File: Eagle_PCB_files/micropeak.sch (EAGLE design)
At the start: 10 parts, among them U1 ATTINY85-20MUR, U2 MS5611-01BA03

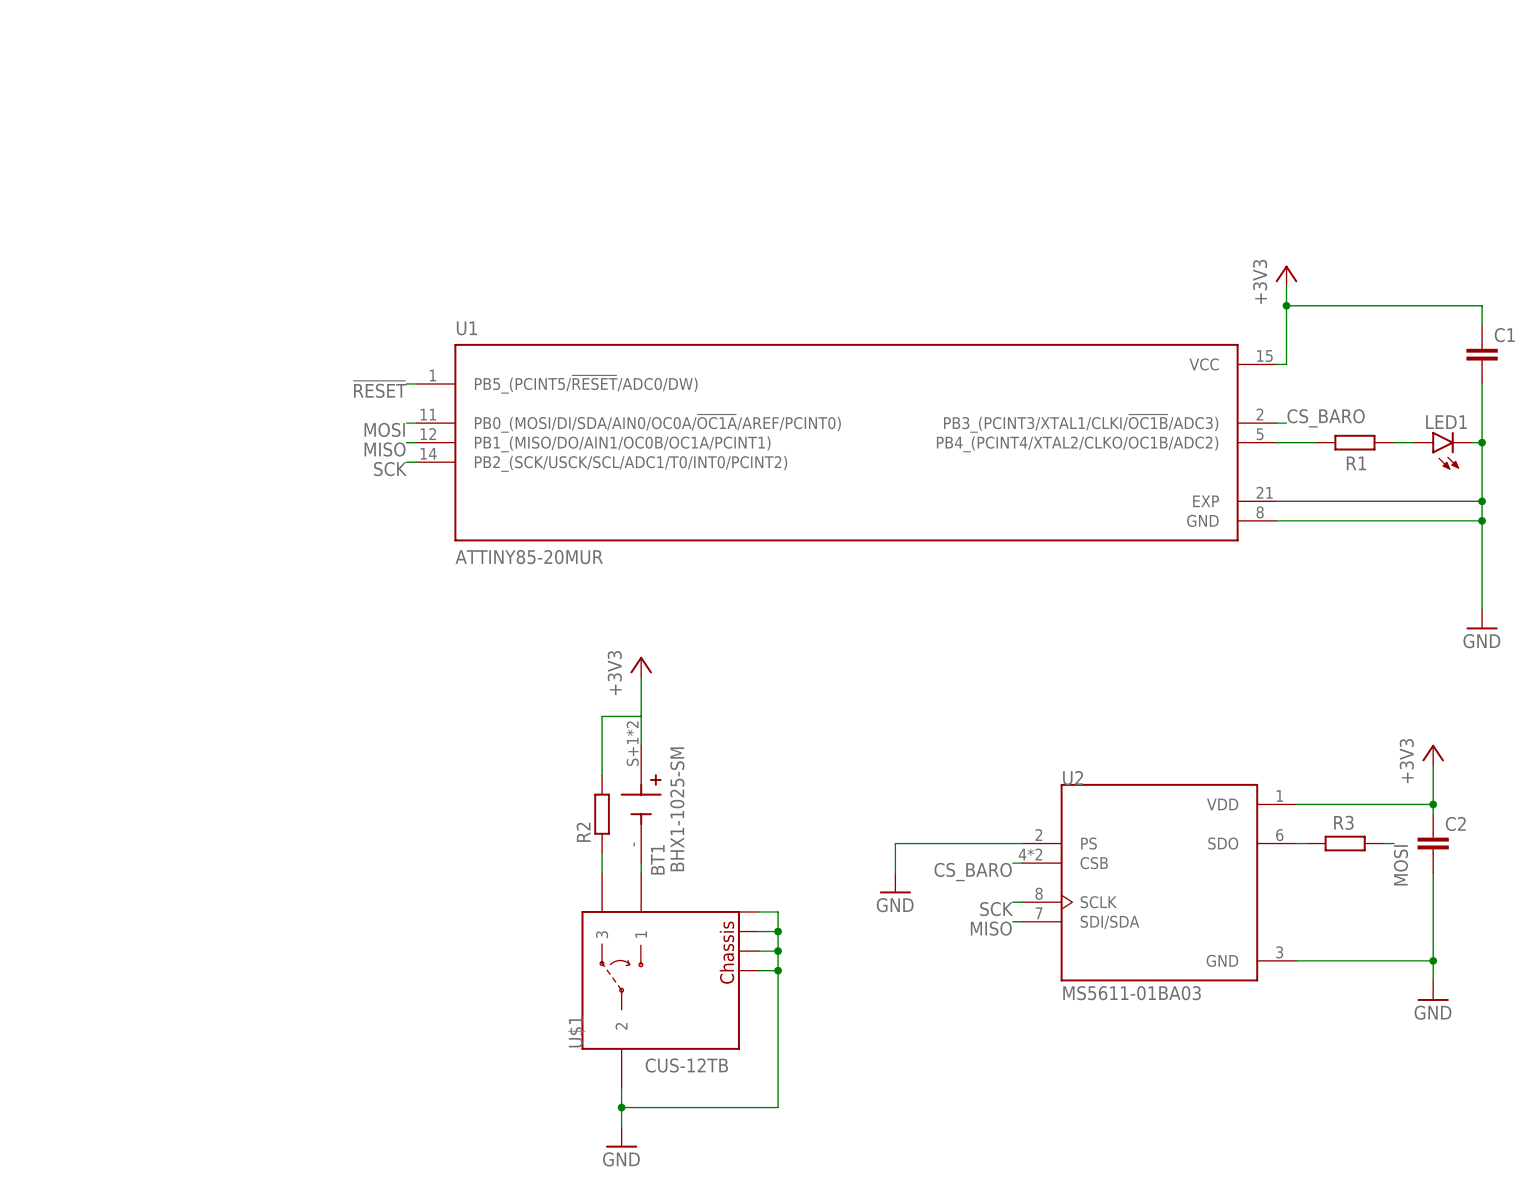
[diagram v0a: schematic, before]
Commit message: schematic done
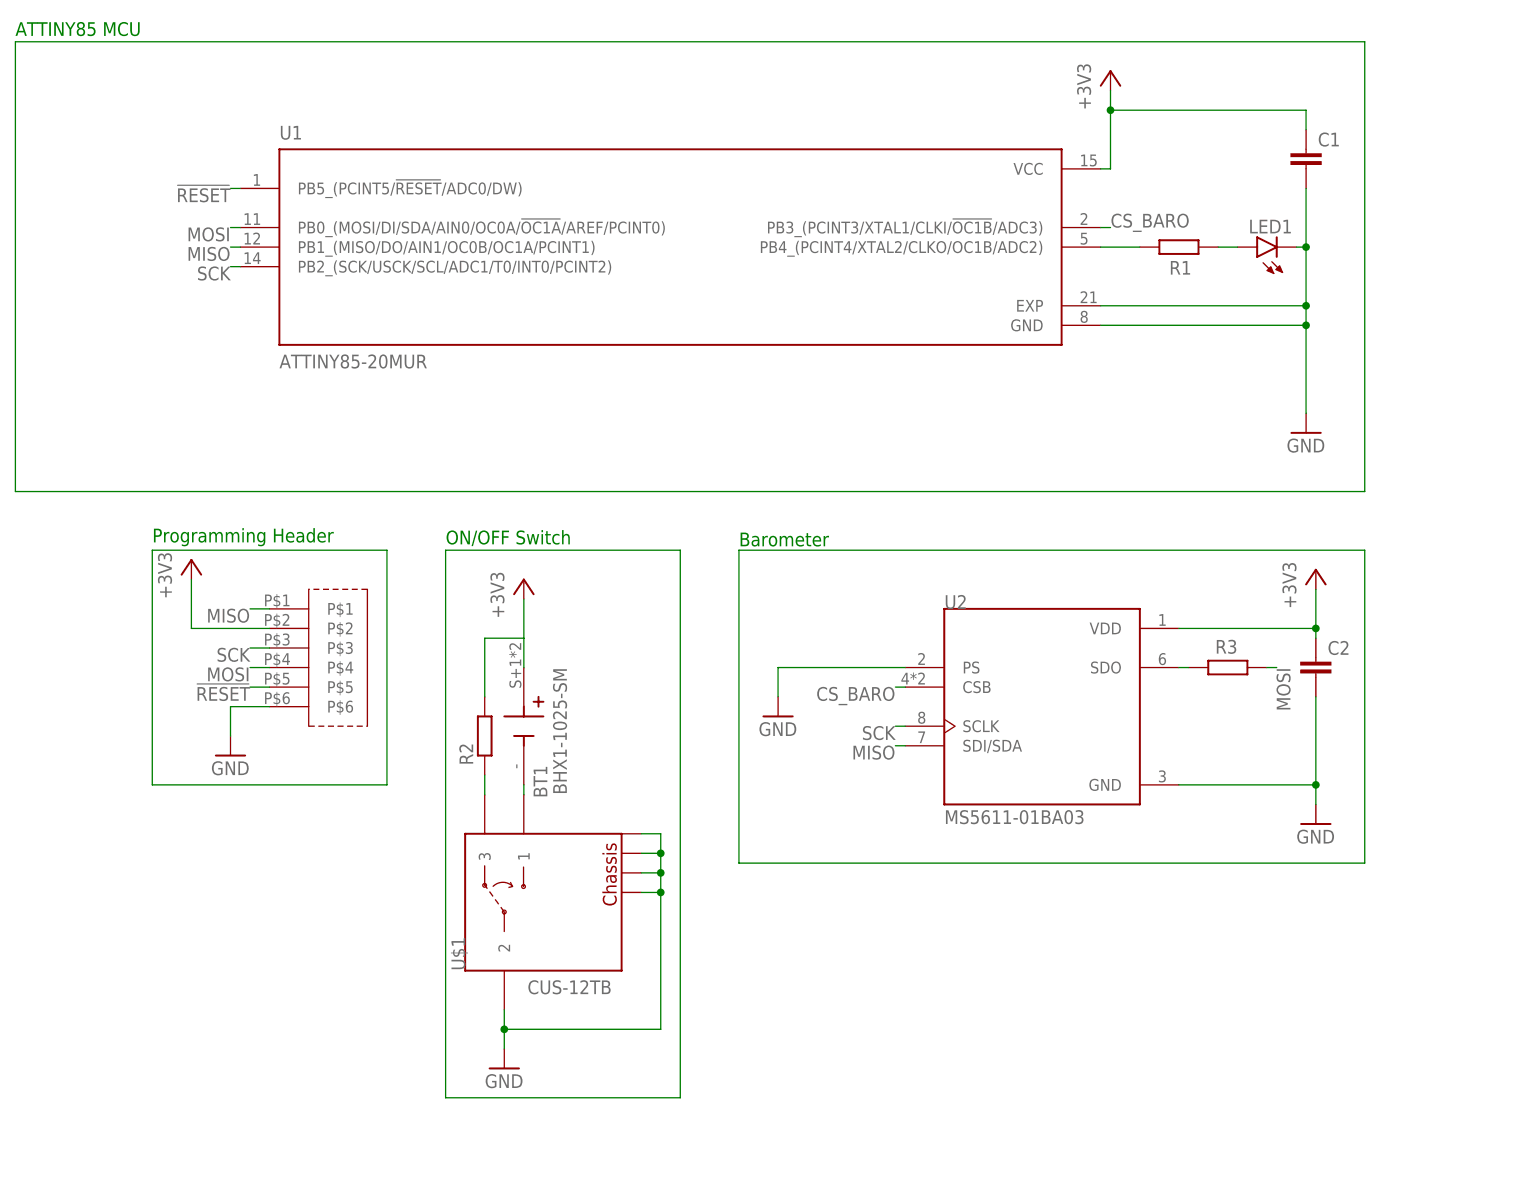
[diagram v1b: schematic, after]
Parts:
- added U$2: 1X6_PROG_HEADER, 1x6_prog_header:1X6_PROG_HEADER
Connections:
- net !RESET!: now also U$2.P$5
- net +3V3: now also U$2.P$2
- net GND: now also U$2.P$6
- net MISO: now also U$2.P$1
- net MOSI: now also U$2.P$4
- net SCK: now also U$2.P$3
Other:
- note added: "ATTINY85 MCU"
- note added: "Barometer"
- note added: "ON/OFF Switch"
- note added: "Programming Header"
- moved on the sheet: BT1, C1, C2, LED1, R1, R2, R3, U$1, U1, U2
